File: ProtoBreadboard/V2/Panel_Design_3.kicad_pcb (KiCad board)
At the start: 2 copper layers, 120.8 x 42.6 mm, 58 parts, among them IC2 BSS138, IC3 BSS138, IC4 BSS138, IC5 BSS138, J10 Conn_01x04_Female, J11 Conn_01x02_Female, J12 Conn_01x02_Female, J13 Conn_01x02_Female, J15 Conn_01x04_Female, J16 Conn_01x03_Female, J17 Conn_01x03_Female, J19 Conn_01x02_Female, J20 Conn_01x02_Female, J21 Conn_01x02_Female, J22 AVR-ISP-6, J23 Conn_01x02_Female, J24 Conn_01x03_Female, J26 Conn_01x03_Female, J27 Conn_02x03_Counter_Clockwise, J28 Conn_01x03_Female, J29 Conn_01x02_Female, J30 Conn_01x02_Female, J31 Conn_01x02_Female, J32 Conn_01x02_Female, J33 Conn_01x03_Female, J34 Conn_01x02_Female, J35 Conn_01x04_Female, J36 Conn_01x02_Female, J6 Conn_01x02_Female, J7 Conn_01x02_Female, J8 Conn_01x02_Female, J9 Conn_01x04_Female, U2 AP2112K-3.3, U3 PRTR5V0U2X, U4 AP2112K-3.3, Y1 Crystal, Y2 Crystal, Y3 Crystal

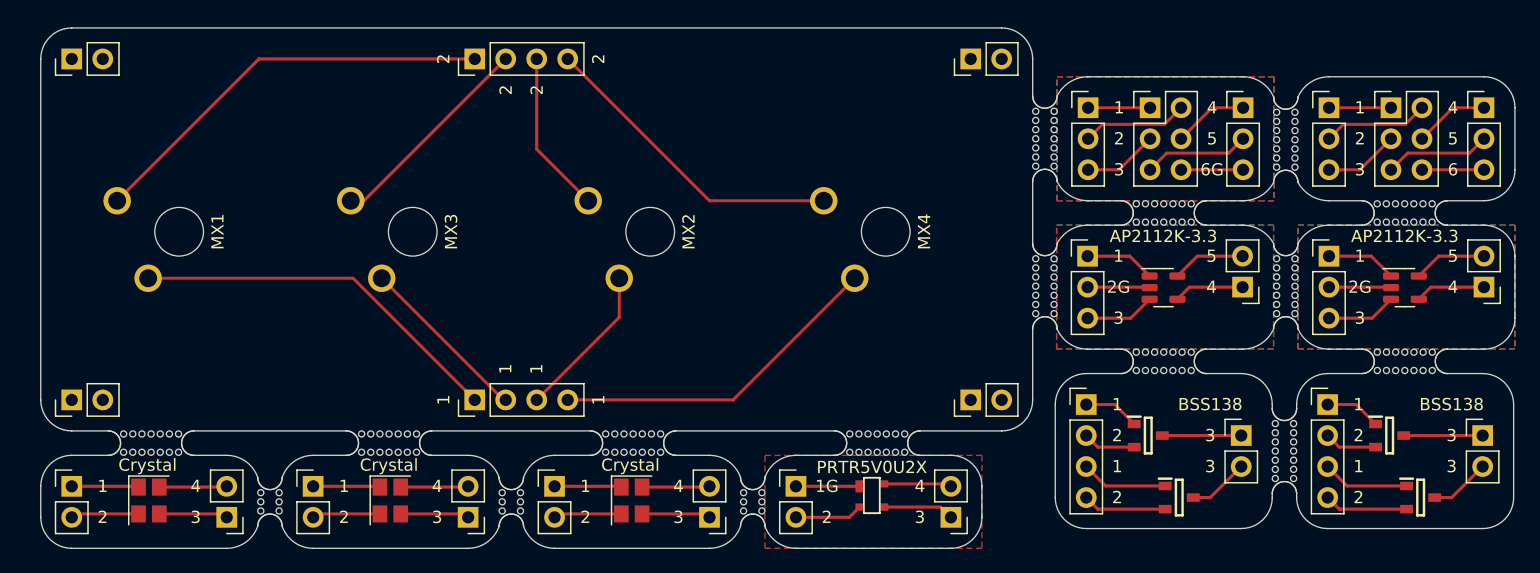
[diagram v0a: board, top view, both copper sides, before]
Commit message: Added Gerber Files for all 3 new designs
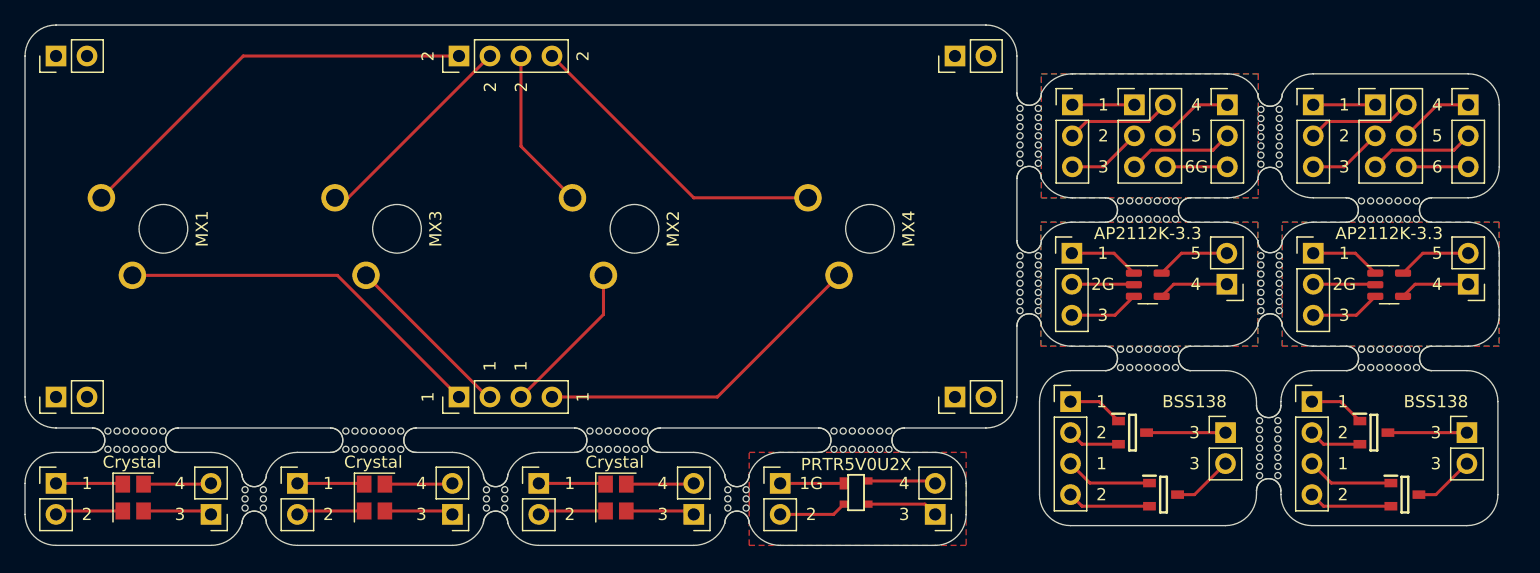
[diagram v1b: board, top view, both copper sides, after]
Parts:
- moved J28 1.31 mm to (146.2, 32.5)
- moved J34 1.31 mm to (146.2, 47.2)
- moved mouse-bite-2mm-slot 1.31 mm to (139.7, 41.1)
- moved mouse-bite-2mm-slot 1.31 mm to (129.9, 60.6)
- moved IC5 1.31 mm to (141.0, 64.4)
- moved J35 1.31 mm to (133.4, 56.8)
- moved Y1 1.31 mm to (36.8, 64.7)
- moved Y3 1.31 mm to (76.4, 64.7)
- moved mouse-bite-2mm-slot 1.31 mm to (66.5, 64.8)
- moved IC2 1.31 mm to (118.7, 59.3)
- moved J16 1.31 mm to (113.7, 44.6)
- moved J19 1.31 mm to (89.8, 63.5)
- moved J24 1.31 mm to (126.5, 32.5)
- moved MX2 1.31 mm to (77.9, 42.6)
- moved U2 1.31 mm to (119.9, 47.2)
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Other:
- outline, holes or cut-outs redrawn
